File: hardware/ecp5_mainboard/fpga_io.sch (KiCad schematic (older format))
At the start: 74 parts, among them J10 UART, J11 FLASH, J12 JTAG, J5 EXT0, J6 EXT1, J7 EXT1, J8 EXT1, J9 PMOD_01, Q9 BSH111BKR, SW6 SW_Push, U15 ECP5UM5G_85_CABGA756, U26 XL_XO_LVDS, U27 W25Q

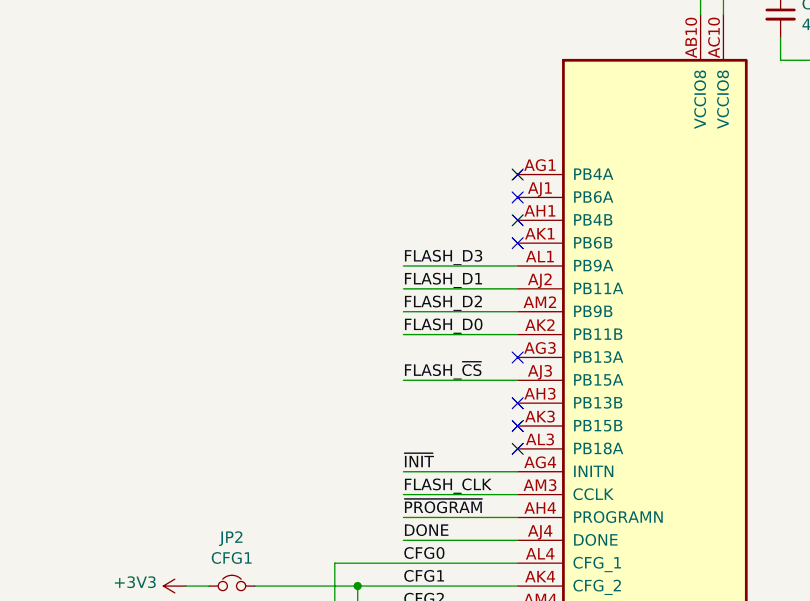
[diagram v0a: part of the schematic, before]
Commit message: hardware/mainboard: add microSD
Signed-off-by: David Shah <dave@ds0.me>
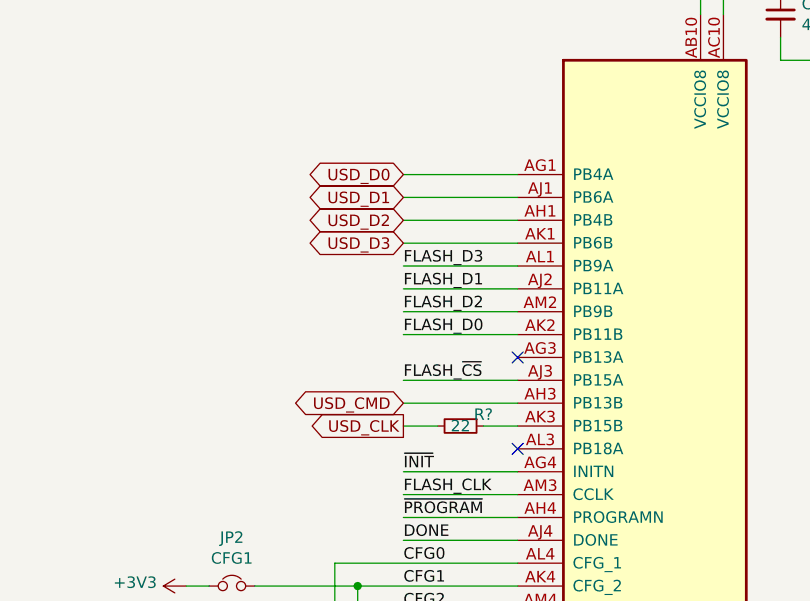
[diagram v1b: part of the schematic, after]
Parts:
- added R?: 22, symbol Device:R_Small
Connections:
- net USD_D0: now reaches U15.AG1 (PB4A)
- net USD_D2: now reaches U15.AH1 (PB4B)
- net USD_CMD: now reaches U15.AH3 (PB13B)
- net USD_D1: now reaches U15.AJ1 (PB6A)
- net USD_D3: now reaches U15.AK1 (PB6B)
- net at U15.AK3 (PB15B): now also R?.1
- new net USD_CLK: R?.2
- no-connect marks 70 -> 64
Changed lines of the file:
@@
 NoConn ~ 5600 8100
 NoConn ~ 5600 8200
-NoConn ~ 20650 4600
-NoConn ~ 20650 4700
-NoConn ~ 20650 4800
-NoConn ~ 20650 4900
 NoConn ~ 20650 5400
-NoConn ~ 20650 5600
-NoConn ~ 20650 5700
 NoConn ~ 20650 5800
 NoConn ~ 8100 11700
@@
 Wire Wire Line
 	11850 6900 11500 6900
+Text GLabel 20150 4600 0    50   BiDi ~ 0
+USD_D0
+Text GLabel 20150 4700 0    50   BiDi ~ 0
+USD_D1
+Text GLabel 20150 4800 0    50   BiDi ~ 0
+USD_D2
+Text GLabel 20150 4900 0    50   BiDi ~ 0
+USD_D3
+Text GLabel 20150 5600 0    50   BiDi ~ 0
+USD_CMD
+Text GLabel 20150 5700 0    50   Output ~ 0
+USD_CLK
+Wire Wire Line
+	20650 5600 20150 5600
+Wire Wire Line
+	20150 4900 20650 4900
+Wire Wire Line
+	20650 4800 20150 4800
+Wire Wire Line
+	20150 4700 20650 4700
+Wire Wire Line
+	20650 4600 20150 4600
+$Comp
+L Device:R_Small R?
+U 1 1 630CCB0A
+P 20400 5700
+F 0 "R?" V 20350 5800 50  0000 C CNN
+F 1 "22" V 20400 5700 50  0000 C CNN
+F 2 "" H 20400 5700 50  0001 C CNN
+F 3 "~" H 20400 5700 50  0001 C CNN
+	1    20400 5700
+	0    1    1    0
+$EndComp
+Wire Wire Line
+	20500 5700 20650 5700
+Wire Wire Line
+	20300 5700 20150 5700
 $EndSCHEMATC
